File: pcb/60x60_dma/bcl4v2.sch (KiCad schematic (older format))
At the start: 43 parts, among them Q1 BSS138, SW1 SW_Push, SW2 SW_Push, SW3 SW_Push, U1 DS9166A-23, U2 STM32F070CBTx, Y1 Resonator, Y2 ABS07-120-32.768kHz-T

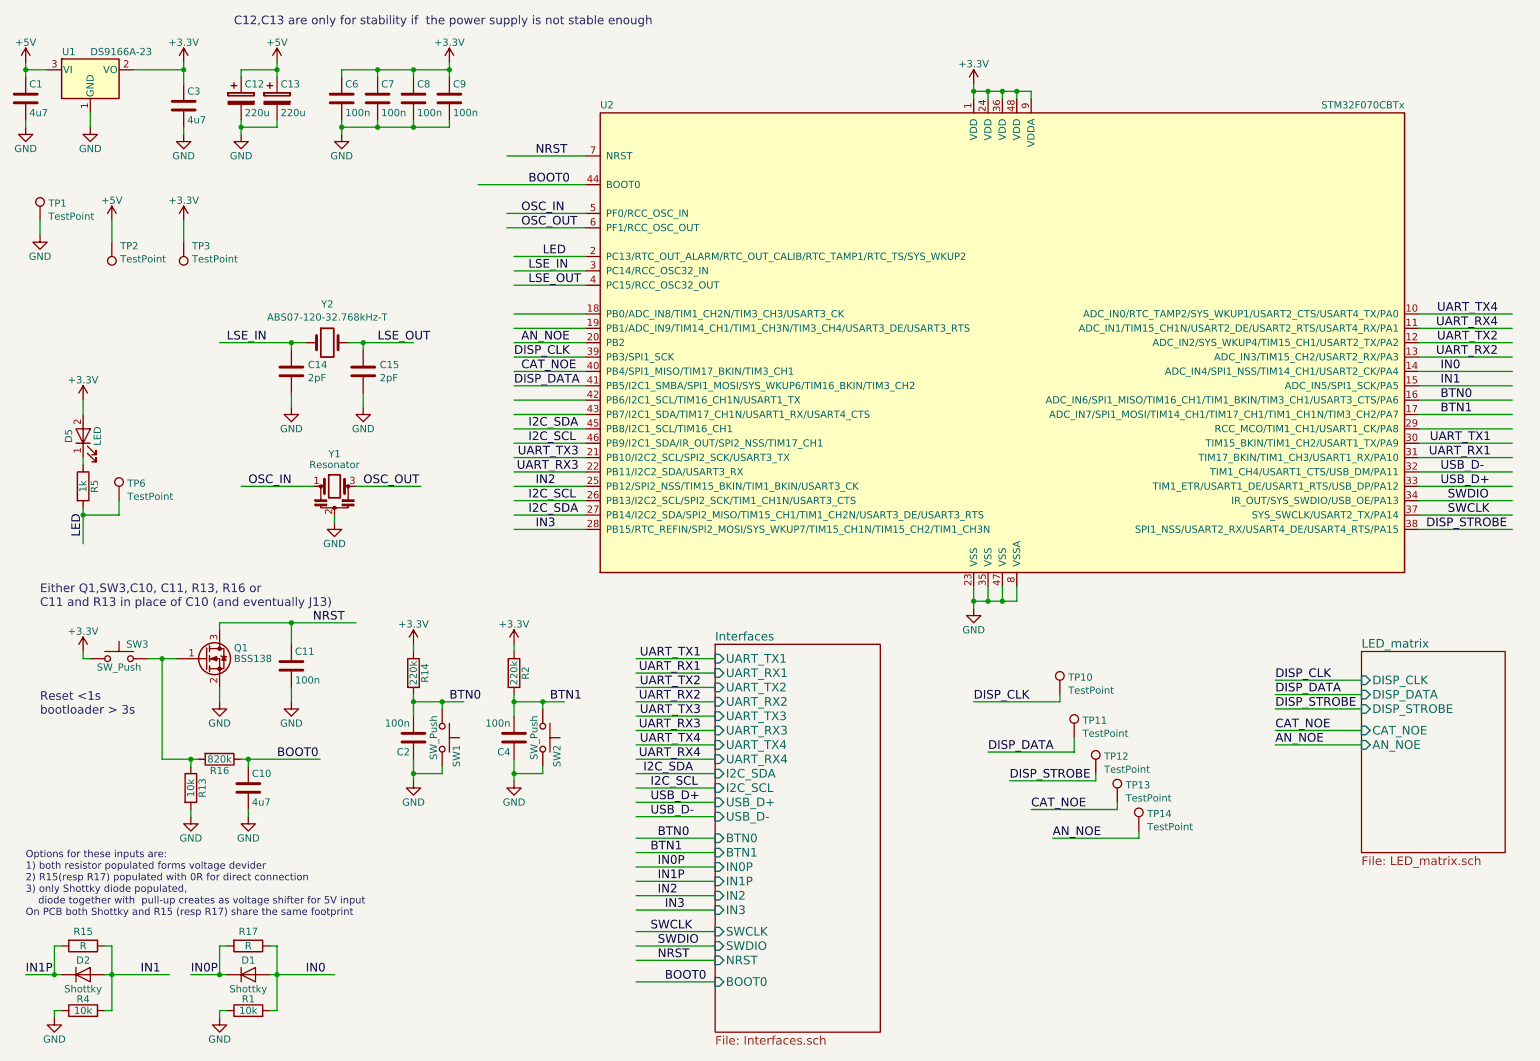
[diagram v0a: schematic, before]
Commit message: - clense the schematics
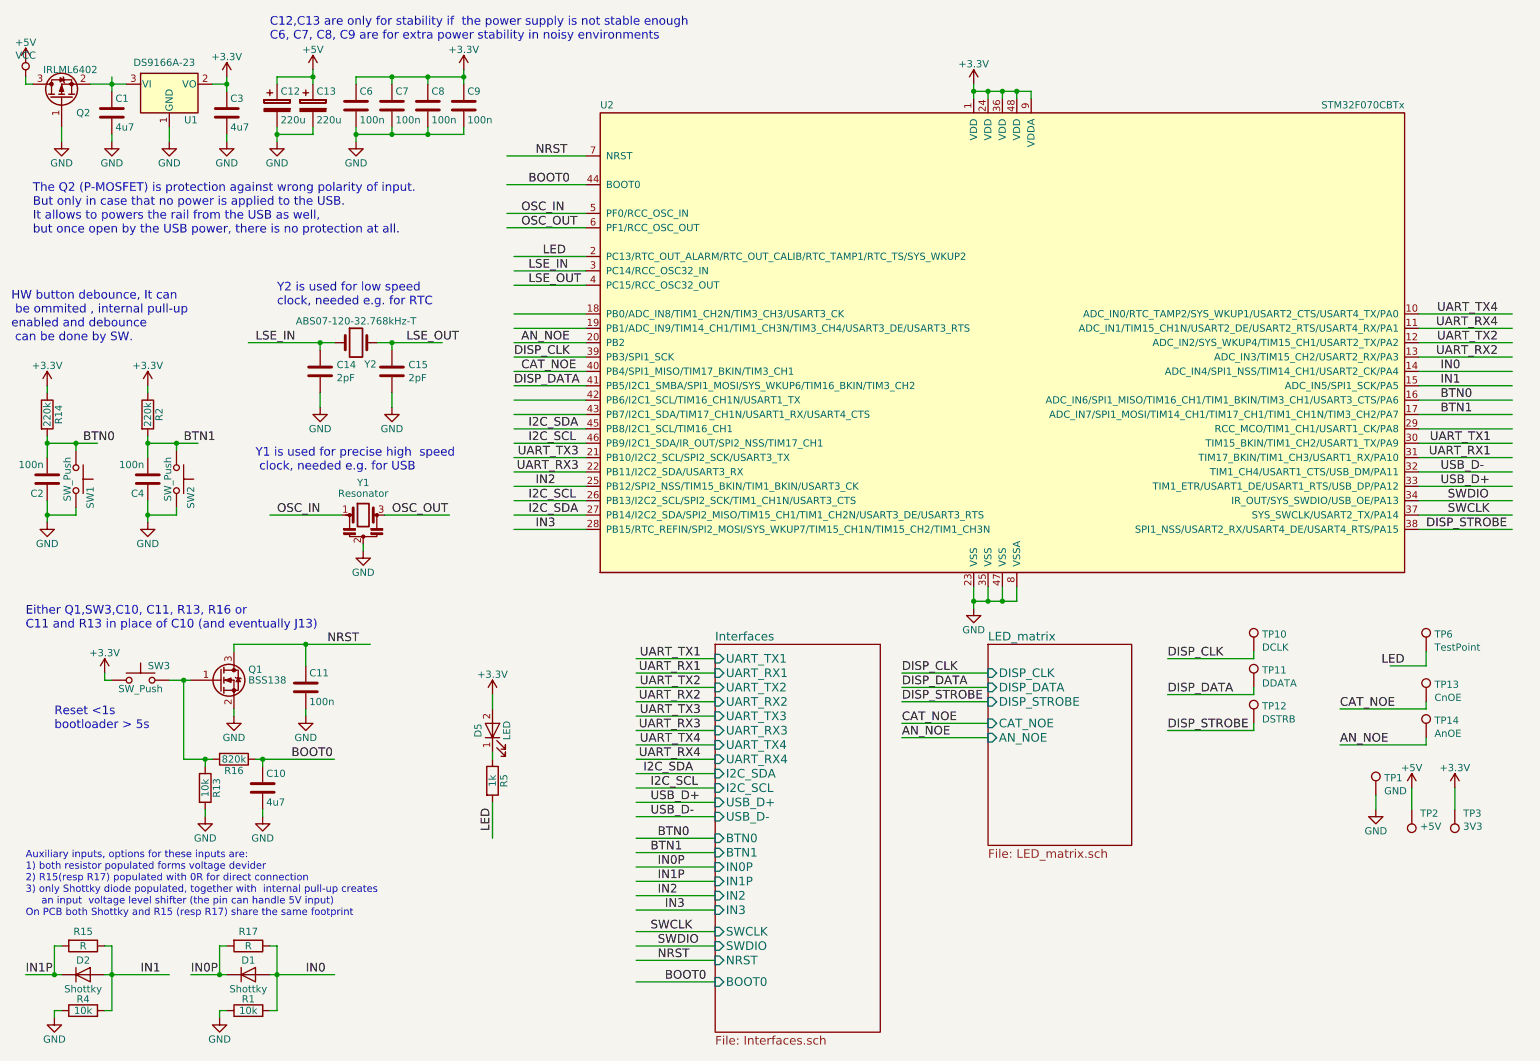
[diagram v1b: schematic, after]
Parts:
- added Q2: IRLML6402, kicad_libraries_new:badger_SOT-23_handsolder, symbol bcl4v2-rescue:Q_PMOS_GSD
- TP1: value TestPoint -> GND
- TP10: value TestPoint -> DCLK
- TP11: value TestPoint -> DDATA
- TP12: value TestPoint -> DSTRB
- TP13: value TestPoint -> CnOE
- TP14: value TestPoint -> AnOE
- TP2: value TestPoint -> +5V
- TP3: value TestPoint -> 3V3
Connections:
- net labels added: VCC
- wire segments 210 -> 213
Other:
- note added: "Auxiliary inputs, options for these inputs are:\n1) both resistor populated forms voltage devider\n2) R15(resp R17) populated with 0R for direct connection\n3) only Shottky diode populated, together with internal pull-up creates\n an input voltage level shifter (the pin can handle 5V input)\nOn PCB both Shottky and R15 (resp R17) share the same footprint\n"
- note added: "C12,C13 are only for stability if the power supply is not stable enough\nC6, C7, C8, C9 are for extra power stability in noisy environments"
- note added: "HW button debounce, It can\n be ommited , internal pull-up\nenabled and debounce\n can be done by SW."
- note added: "Reset <1s\nbootloader > 5s"
- note added: "The Q2 (P-MOSFET) is protection against wrong polarity of input.\nBut only in case that no power is applied to the USB.\nIt allows to powers the rail from the USB as well,\nbut once open by the USB power, there is no protection at all."
- note added: "Y1 is used for precise high speed\n clock, needed e.g. for USB"
- note added: "Y2 is used for low speed \nclock, needed e.g. for RTC"
- note removed: "C12,C13 are only for stability if the power supply is not stable enough"
- note removed: "Options for these inputs are:\n1) both resistor populated forms voltage devider\n2) R15(resp R17) populated with 0R for direct connection\n3) only Shottky diode populated, \n diode together with pull-up creates as voltage shifter for 5V input\nOn PCB both Shottky and R15 (resp R17) share the same footprint\n"
- note removed: "Reset <1s\nbootloader > 3s"
- moved on the sheet: C1, C10, C11, C12, C13, C14, C15, C2, C3, C4, C6, C7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
